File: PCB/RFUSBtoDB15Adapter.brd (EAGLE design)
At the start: 52.1 x 68.6 mm, 24 parts, among them IC1 S-816A40AMC-BAPT2U, J1 0, J2 AVR_SPI_PROG_3X2NS, Q2 2SA1213-Y(TE12L,F)

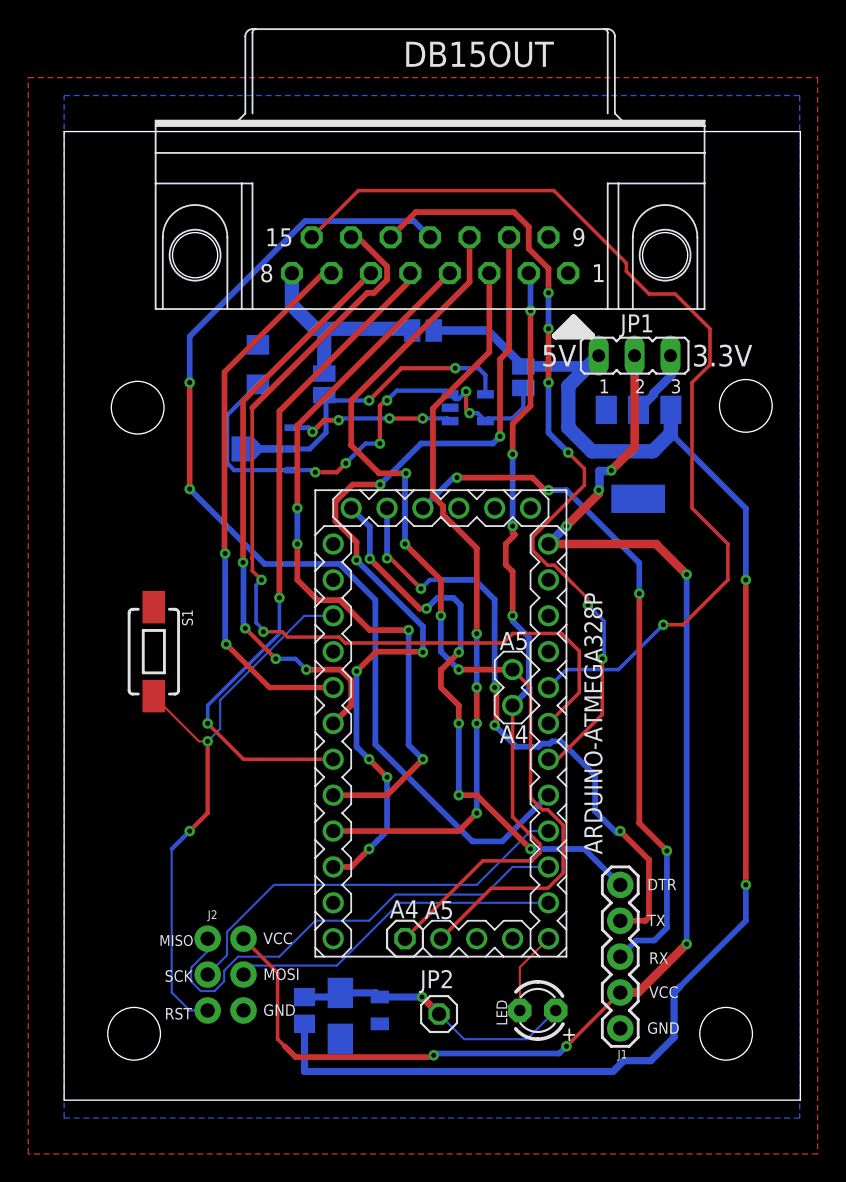
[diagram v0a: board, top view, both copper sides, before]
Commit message: PCB
PCB design updated
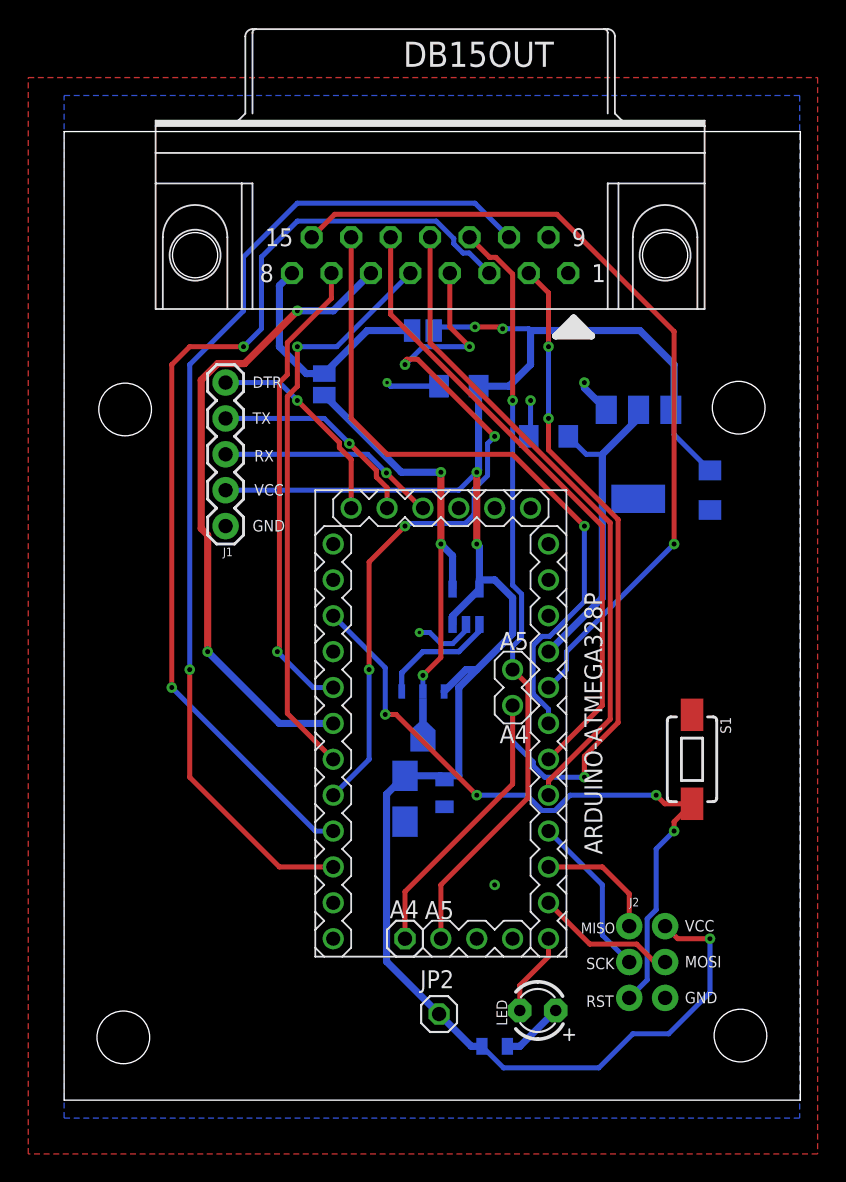
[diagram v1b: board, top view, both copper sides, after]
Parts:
- removed JP1: (no value), jumper:JP2
- removed SJ3: (no value), jumper:SJ
- added C3, C4: 10uF, SparkFun-Capacitors:EIA3216
- R1: value 33Ω -> 80R; device eagle-ltspice:R0805 -> SparkFun-Resistors:0805
- moved J1 45.2 mm to (8.89, 52.1)
- moved S1 38.9 mm to (41.9, 35.6)
- moved J2 29.9 mm to (38.7, 21.2)
- moved Q2 21.9 mm to (22.9, 38.6), turned to 180 degrees
- moved C1 16.0 mm to (24.4, 33.1)
- moved C5 16.0 mm to (21.6, 32.8)
- moved C2 14.3 mm to (25.4, 62.0), turned to 180 degrees
- moved IC1 14.1 mm to (25.9, 46.4), turned to 90 degrees
- moved R1 13.7 mm to (27.9, 15.2), turned to 0 degrees
- moved PEM2 1.02 mm to (45.3, 16.0)
- moved PEM3 0.90 mm to (1.78, 60.3)
- moved PEM1 0.80 mm to (1.65, 15.9)
- moved PEM4 0.52 mm to (45.2, 60.5)
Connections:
- removed net VBUS: C1.2, C5.+, JP2.1, LED.A, R1.1
- removed net VCC: ARDUINO-ATMEGA328P.J6.4
- removed net VCCIN: ARDUINO-ATMEGA328P.J6.1, J1.2, J2.2, JP1.2
- new net 5VLED: LED.A, R1.1
- new net RAW: ARDUINO-ATMEGA328P.J6.1
- net 3.3V: now also ARDUINO-ATMEGA328P.J6.4, C4.+; no longer JP1.3
- net 5VREG: now also C1.2, C3.+, C5.+, J1.2, J2.2, JP2.1; no longer JP1.1, SJ3.1, SJ3.2
- net GND: now also C3.-, C4.-
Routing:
- net VCCIN: track 94.1 -> 0.00 mm, vias 7 -> 0
- net RX: track 49.5 -> 15.5 mm, vias 4 -> 1
- net TX: track 44.9 -> 15.2 mm, vias 5 -> 1
- net BUT3: track 74.8 -> 46.6 mm, vias 2 -> 0
- net DTR: track 41.2 -> 14.8 mm, vias 6 -> 1
- net MISO: track 33.2 -> 8.79 mm
- net VBUS: track 20.1 -> 0.00 mm, vias 1 -> 0
- net CREDIT: track 51.8 -> 69.9 mm, vias 4 -> 2
- net 3.3V: track 4.82 -> 22.7 mm
- net SCK: track 29.3 -> 11.6 mm
- net LEFT: track 63.6 -> 48.7 mm, vias 2 -> 1
- net START: track 68.9 -> 54.7 mm, vias 4 -> 1
- net MOSI: track 23.8 -> 9.99 mm
- net GND: track 0.00 -> 13.4 mm, vias 0 -> 5
- net 5VSG: track 34.2 -> 47.1 mm, vias 2 -> 3
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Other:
- board text removed: "3.3V"
- board text removed: "5V"
